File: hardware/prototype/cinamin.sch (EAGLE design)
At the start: 115 parts, among them J1 INPUT_DIVIDER, J10 TO_BLE, J11 TO_ADM, J12 INPUT_DIVIDER, J13 TO_LTC1540, J14 STAGE_1_PULL, J15 TO_AP440, J16 STAGE_2_PULL, J17 OFF_DIVIDER, J18 TO_BLE, J19 TO_AP440, J20 TO_BLE, J21 TO_BQ25504, J22 TO_BLE, J3 TO_ADM2, J4 TO_ADM1, J5 TO_LATCH, J6 STAGE_1_PULL, J7 STAGE_2_PULL, J8 OFF_DIVIDER, J9 TO_BLE, Q2 MOSFET-NCHANNELXFDN-3, Q5 MOSFET-NCHANNELXFDN-3, Q8 MOSFET-NCHANNELXFDN-3, U1 LTC1540, U5 ltc1540, U6 AP4400_3.4_2.3, U7 BQ25504RGT, U8 DA14580, X1 16Mhz, X2 16Mhz

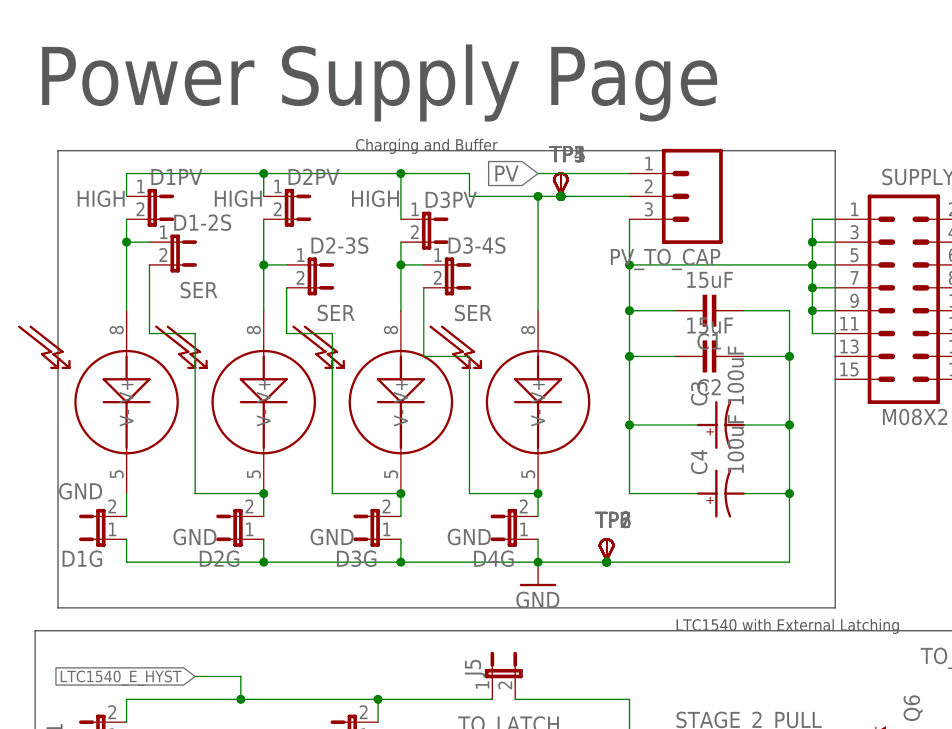
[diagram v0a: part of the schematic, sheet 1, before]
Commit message: committing board sent to fab
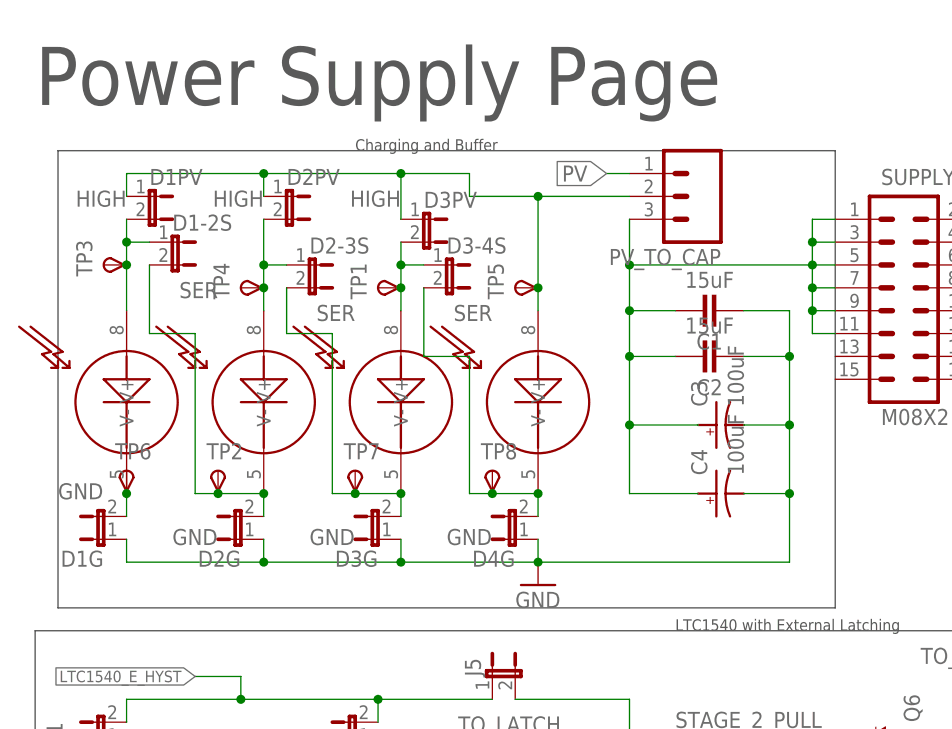
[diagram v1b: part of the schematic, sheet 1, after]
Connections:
- net GND: no longer TP2.PP, TP6.PP, TP7.PP, TP8.PP
- net N$43: now also TP8.PP
- net N$61: now also TP6.PP
- net N$62: now also TP2.PP
- net N$63: now also TP7.PP
- net N$65: now also TP3.PP
- net N$66: no longer TP1.PP, TP3.PP, TP4.PP
- net N$67: now also TP4.PP
- net N$68: now also TP1.PP
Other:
- moved on the sheet: TP1, TP2, TP3, TP4, TP5, TP6, TP7, TP8
